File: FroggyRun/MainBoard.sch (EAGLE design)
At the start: 17 parts

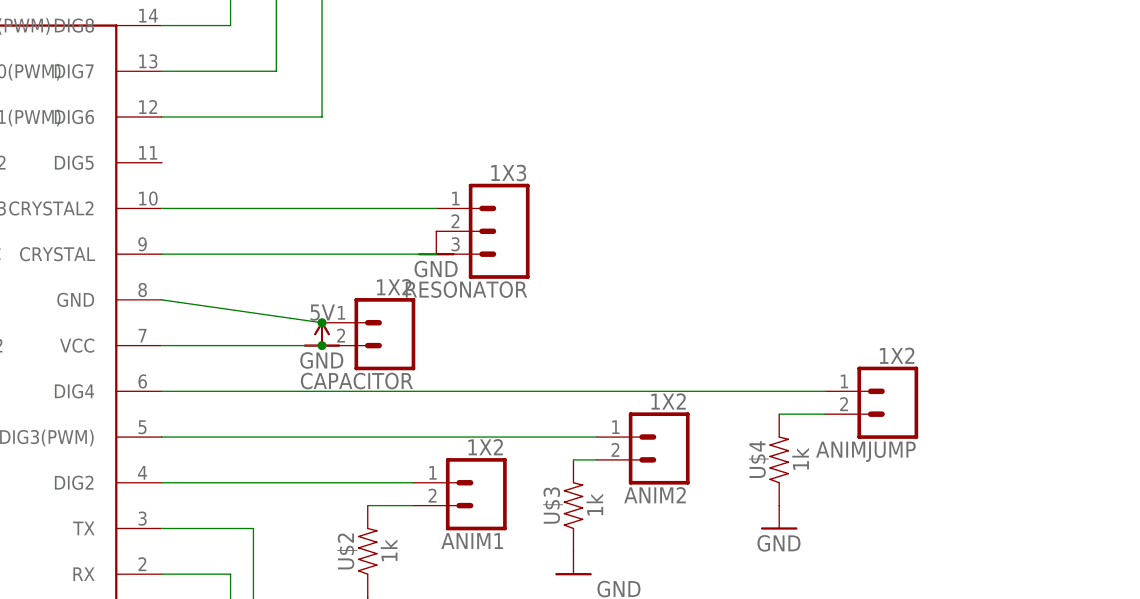
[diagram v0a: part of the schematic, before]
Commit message: hjk
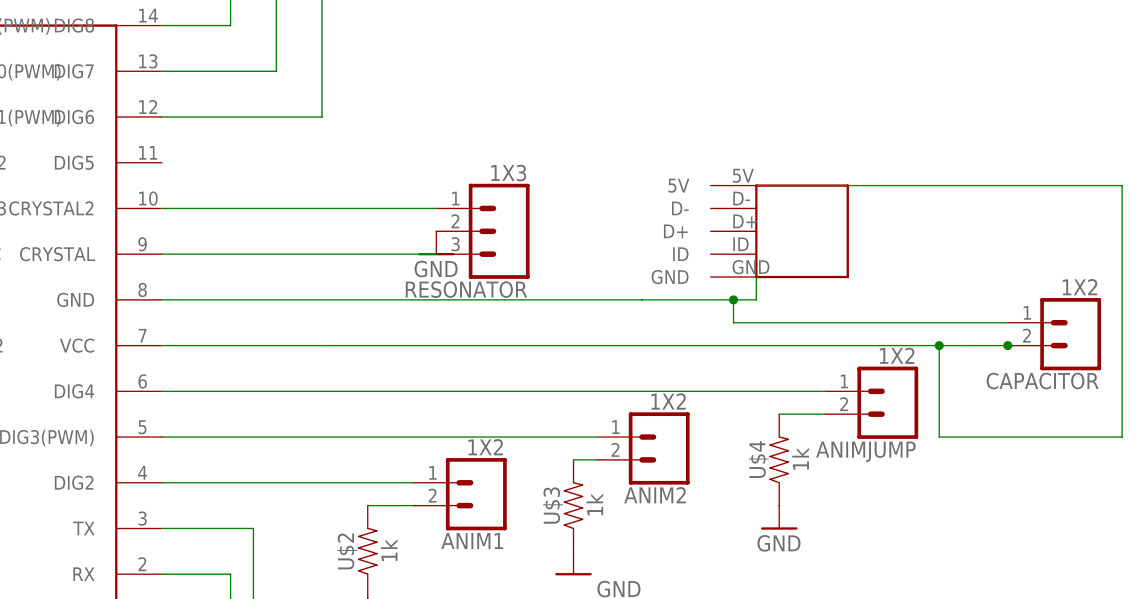
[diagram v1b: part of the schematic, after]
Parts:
- added U$8: USB, FroggyRun:USB
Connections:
- new net N$20: CAPACITOR.1, U$1.GND, U$8.GND
- new net N$21: CAPACITOR.2, U$1.VCC, U$8.5V
- net GND: no longer CAPACITOR.1, U$1.GND
- net VIN: no longer CAPACITOR.2, U$1.VCC
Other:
- moved on the sheet: CAPACITOR
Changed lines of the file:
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@@
 <part name="GND5" library="supply1" library_urn="urn:adsk.eagle:library:371" deviceset="GND" device=""/>
 <part name="GND6" library="supply1" library_urn="urn:adsk.eagle:library:371" deviceset="GND" device=""/>
-<part name="5V2" library="SparkFun-PowerSymbols" library_urn="urn:adsk.eagle:library:530" deviceset="VIN" device="" value="5V"/>
 <part name="5V3" library="SparkFun-PowerSymbols" library_urn="urn:adsk.eagle:library:530" deviceset="VIN" device="" value="5V"/>
 <part name="GND7" library="supply1" library_urn="urn:adsk.eagle:library:371" deviceset="GND" device=""/>
@@
 <part name="U$1" library="FroggyRun" deviceset="ATMEGA328" device=""/>
 <part name="PROGRAMMING" library="FroggyRun" deviceset="1X6" device=""/>
-<part name="GND1" library="supply1" library_urn="urn:adsk.eagle:library:371" deviceset="GND" device=""/>
 <part name="5V4" library="SparkFun-PowerSymbols" library_urn="urn:adsk.eagle:library:530" deviceset="VIN" device="" value="5V"/>
 <part name="5V5" library="SparkFun-PowerSymbols" library_urn="urn:adsk.eagle:library:530" deviceset="VIN" device="" value="5V"/>
@@
 <part name="GND12" library="supply1" library_urn="urn:adsk.eagle:library:371" deviceset="GND" device=""/>
 <part name="U$7" library="FroggyRun" deviceset="BUTTON" device=""/>
+<part name="U$8" library="FroggyRun" deviceset="USB" device=""/>
 </parts>
 <sheets>
@@
 <attribute name="VALUE" x="91.44" y="35.56" size="1.778" layer="96"/>
 </instance>
-<instance part="5V2" gate="G$1" x="88.9" y="68.58" smashed="yes">
-<attribute name="VALUE" x="88.9" y="71.374" size="1.778" layer="96" align="bottom-center"/>
-</instance>
 <instance part="5V3" gate="G$1" x="73.66" y="147.32" smashed="yes">
 <attribute name="VALUE" x="73.66" y="150.114" size="1.778" layer="96" align="bottom-center"/>
@@
 <attribute name="NAME" x="99.06" y="12.192" size="1.778" layer="95" font="vector" rot="R180"/>
 </instance>
-<instance part="GND1" gate="1" x="88.9" y="68.58" smashed="yes">
-<attribute name="VALUE" x="86.36" y="66.04" size="1.778" layer="96"/>
-</instance>
 <instance part="5V4" gate="G$1" x="15.24" y="86.36" smashed="yes">
 <attribute name="VALUE" x="15.24" y="89.154" size="1.778" layer="96" align="bottom-center"/>
@@
 <attribute name="NAME" x="111.76" y="75.692" size="1.778" layer="95" font="vector" rot="R180"/>
 </instance>
-<instance part="CAPACITOR" gate="G$1" x="96.52" y="71.12" smashed="yes" rot="R180">
-<attribute name="VALUE" x="99.06" y="75.946" size="1.778" layer="96" font="vector" rot="R180"/>
-<attribute name="NAME" x="99.06" y="65.532" size="1.778" layer="95" font="vector" rot="R180"/>
+<instance part="CAPACITOR" gate="G$1" x="172.72" y="71.12" smashed="yes" rot="R180">
+<attribute name="VALUE" x="175.26" y="75.946" size="1.778" layer="96" font="vector" rot="R180"/>
+<attribute name="NAME" x="175.26" y="65.532" size="1.778" layer="95" font="vector" rot="R180"/>
 </instance>
 <instance part="GND12" gate="1" x="101.6" y="78.74" smashed="yes">
@@
 </instance>
 <instance part="U$7" gate="G$1" x="45.72" y="10.16" smashed="yes"/>
+<instance part="U$8" gate="G$1" x="142.24" y="81.28" smashed="yes" rot="R180"/>
 </instances>
 <busses>
@@
 </segment>
 <segment>
-<pinref part="U$1" gate="G$1" pin="GND"/>
-<pinref part="GND1" gate="1" pin="GND"/>
-<wire x1="71.12" y1="73.66" x2="88.9" y2="71.12" width="0.1524" layer="91"/>
-<pinref part="CAPACITOR" gate="G$1" pin="1"/>
-<junction x="88.9" y="71.12"/>
-</segment>
-<segment>
 <pinref part="LEDSTRIP" gate="G$1" pin="1"/>
 <wire x1="-2.54" y1="91.44" x2="-2.54" y2="86.36" width="0.1524" layer="91"/>
@@
 <pinref part="5V1" gate="G$1" pin="VIN"/>
 <wire x1="40.64" y1="78.74" x2="35.56" y2="78.74" width="0.1524" layer="91"/>
-</segment>
-<segment>
-<pinref part="U$1" gate="G$1" pin="VCC"/>
-<wire x1="71.12" y1="68.58" x2="88.9" y2="68.58" width="0.1524" layer="91"/>
-<pinref part="5V2" gate="G$1" pin="VIN"/>
-<pinref part="CAPACITOR" gate="G$1" pin="2"/>
-<junction x="88.9" y="68.58"/>
 </segment>
 <segment>
@@
 </segment>
 </net>
+<net name="N$21" class="0">
+<segment>
+<pinref part="U$1" gate="G$1" pin="VCC"/>
+<wire x1="71.12" y1="68.58" x2="88.9" y2="68.58" width="0.1524" layer="91"/>
+<pinref part="CAPACITOR" gate="G$1" pin="2"/>
+<junction x="165.1" y="68.58"/>
+<wire x1="165.1" y1="68.58" x2="160.02" y2="68.58" width="0.1524" layer="91"/>
+<pinref part="U$8" gate="G$1" pin="5V"/>
+<wire x1="157.48" y1="68.58" x2="88.9" y2="68.58" width="0.1524" layer="91"/>
+<wire x1="137.16" y1="86.36" x2="177.8" y2="86.36" width="0.1524" layer="91"/>
+<wire x1="177.8" y1="86.36" x2="177.8" y2="58.42" width="0.1524" layer="91"/>
+<wire x1="177.8" y1="58.42" x2="157.48" y2="58.42" width="0.1524" layer="91"/>
+<wire x1="157.48" y1="58.42" x2="157.48" y2="68.58" width="0.1524" layer="91"/>
+<wire x1="157.48" y1="68.58" x2="160.02" y2="68.58" width="0.1524" layer="91"/>
+<junction x="157.48" y="68.58"/>
+</segment>
+</net>
+<net name="N$20" class="0">
+<segment>
+<pinref part="U$1" gate="G$1" pin="GND"/>
+<wire x1="71.12" y1="73.66" x2="124.46" y2="73.66" width="0.1524" layer="91"/>
+<wire x1="124.46" y1="73.66" x2="134.62" y2="73.66" width="0.1524" layer="91"/>
+<wire x1="134.62" y1="73.66" x2="134.62" y2="71.12" width="0.1524" layer="91"/>
+<pinref part="CAPACITOR" gate="G$1" pin="1"/>
+<wire x1="134.62" y1="71.12" x2="165.1" y2="71.12" width="0.1524" layer="91"/>
+<pinref part="U$8" gate="G$1" pin="GND"/>
+<wire x1="137.16" y1="76.2" x2="137.16" y2="73.66" width="0.1524" layer="91"/>
+<wire x1="137.16" y1="73.66" x2="134.62" y2="73.66" width="0.1524" layer="91"/>
+<junction x="134.62" y="73.66"/>
+</segment>
+</net>
